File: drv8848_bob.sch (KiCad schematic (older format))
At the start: 1 part, among them J2 Conn_01x24

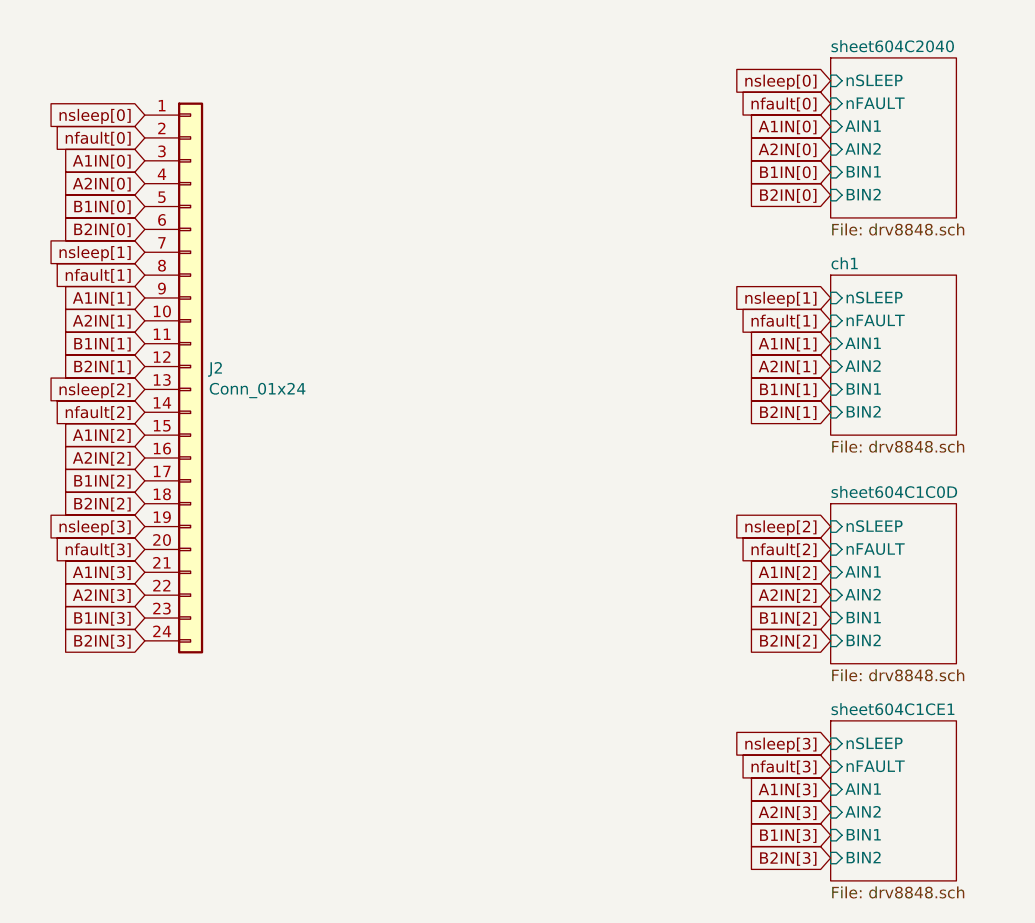
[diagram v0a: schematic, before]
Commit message: finalish
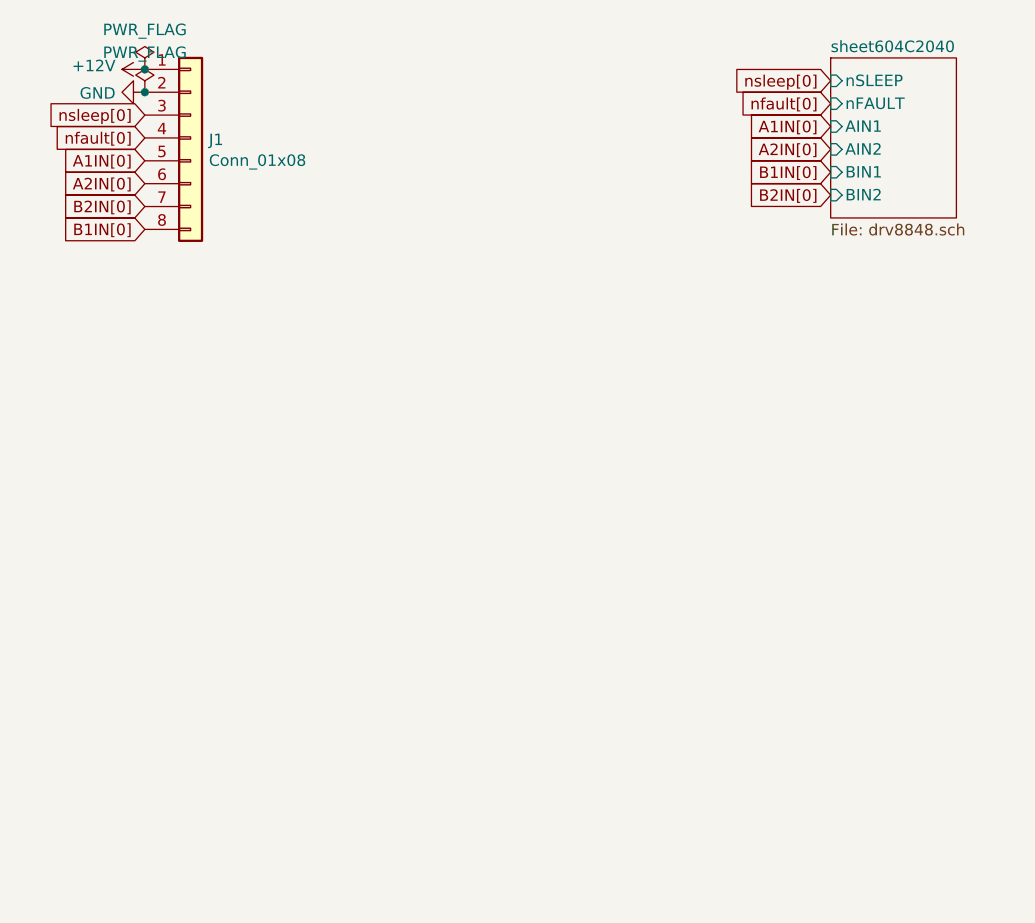
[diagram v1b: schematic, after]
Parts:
- removed J2: Conn_01x24, Connector_PinHeader_2.54mm:PinHeader_1x24_P2.54mm_Vertical, symbol Connector_Generic:Conn_01x24
- added J1: Conn_01x08, Connector_PinHeader_2.54mm:PinHeader_1x08_P2.54mm_Vertical, symbol Connector_Generic:Conn_01x08
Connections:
- net A1IN[0]: now also J1.5 (Pin_5)
- net A2IN[0]: now also J1.6 (Pin_6)
- net B1IN[0]: now also J1.8 (Pin_8)
- net B2IN[0]: now also J1.7 (Pin_7)
- net nfault[0]: now also J1.4 (Pin_4)
- net nsleep[0]: now also J1.3 (Pin_3)
- new net +12V: J1.1 (Pin_1)
- new net GND: J1.2 (Pin_2)
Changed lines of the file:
@@
 $Descr A4 11693 8268
 encoding utf-8
-Sheet 1 5
+Sheet 1 2
 Title ""
 Date ""
@@
 Comment4 ""
 $EndDescr
-$Sheet
-S 8900 2100 550  700
-U 604BEC61
-F0 "ch1" 50
-F1 "drv8848.sch" 50
-F2 "nSLEEP" I L 8900 2200 50
-F3 "nFAULT" I L 8900 2300 50
-F4 "AIN1" I L 8900 2400 50
-F5 "AIN2" I L 8900 2500 50
-F6 "BIN1" I L 8900 2600 50
-F7 "BIN2" I L 8900 2700 50
-$EndSheet
-$Sheet
-S 8900 3100 550  700
-U 604C1C15
-F0 "sheet604C1C0D" 50
-F1 "drv8848.sch" 50
-F2 "nSLEEP" I L 8900 3200 50
-F3 "nFAULT" I L 8900 3300 50
-F4 "AIN1" I L 8900 3400 50
-F5 "AIN2" I L 8900 3500 50
-F6 "BIN1" I L 8900 3600 50
-F7 "BIN2" I L 8900 3700 50
-$EndSheet
-$Sheet
-S 8900 4050 550  700
-U 604C1CE9
-F0 "sheet604C1CE1" 50
-F1 "drv8848.sch" 50
-F2 "nSLEEP" I L 8900 4150 50
-F3 "nFAULT" I L 8900 4250 50
-F4 "AIN1" I L 8900 4350 50
-F5 "AIN2" I L 8900 4450 50
-F6 "BIN1" I L 8900 4550 50
-F7 "BIN2" I L 8900 4650 50
-$EndSheet
 $Sheet
 S 8900 1150 550  700
@@
 Text GLabel 8900 1650 0    50   Input ~ 0
 B1IN[0]
-Text GLabel 8900 2200 0    50   Input ~ 0
-nsleep[1]
-Text GLabel 8900 2300 0    50   Input ~ 0
-nfault[1]
-Text GLabel 8900 2400 0    50   Input ~ 0
-A1IN[1]
-Text GLabel 8900 2500 0    50   Input ~ 0
-A2IN[1]
-Text GLabel 8900 2700 0    50   Input ~ 0
-B2IN[1]
-Text GLabel 8900 2600 0    50   Input ~ 0
-B1IN[1]
-Text GLabel 8900 3200 0    50   Input ~ 0
-nsleep[2]
-Text GLabel 8900 3300 0    50   Input ~ 0
-nfault[2]
-Text GLabel 8900 3400 0    50   Input ~ 0
-A1IN[2]
-Text GLabel 8900 3500 0    50   Input ~ 0
-A2IN[2]
-Text GLabel 8900 3700 0    50   Input ~ 0
-B2IN[2]
-Text GLabel 8900 3600 0    50   Input ~ 0
-B1IN[2]
-Text GLabel 8900 4150 0    50   Input ~ 0
-nsleep[3]
-Text GLabel 8900 4250 0    50   Input ~ 0
-nfault[3]
-Text GLabel 8900 4350 0    50   Input ~ 0
-A1IN[3]
-Text GLabel 8900 4450 0    50   Input ~ 0
-A2IN[3]
-Text GLabel 8900 4650 0    50   Input ~ 0
-B2IN[3]
-Text GLabel 8900 4550 0    50   Input ~ 0
-B1IN[3]
-$Comp
-L Connector_Generic:Conn_01x24 J2
-U 1 1 604C3E6E
-P 6100 2500
-F 0 "J2" H 6180 2492 50  0000 L CNN
-F 1 "Conn_01x24" H 6180 2401 50  0000 L CNN
-F 2 "Connector_PinHeader_2.54mm:PinHeader_1x24_P2.54mm_Vertical" H 6100 2500 50  0001 C CNN
-F 3 "~" H 6100 2500 50  0001 C CNN
-	1    6100 2500
-	1    0    0    -1
-$EndComp
 Text GLabel 5900 1400 0    50   Input ~ 0
 nsleep[0]
@@
 Text GLabel 5900 1700 0    50   Input ~ 0
 A2IN[0]
+Text GLabel 5900 1800 0    50   Input ~ 0
+B2IN[0]
 Text GLabel 5900 1900 0    50   Input ~ 0
-B2IN[0]
-Text GLabel 5900 1800 0    50   Input ~ 0
 B1IN[0]
-Text GLabel 5900 2000 0    50   Input ~ 0
-nsleep[1]
-Text GLabel 5900 2100 0    50   Input ~ 0
-nfault[1]
-Text GLabel 5900 2200 0    50   Input ~ 0
-A1IN[1]
-Text GLabel 5900 2300 0    50   Input ~ 0
-A2IN[1]
-Text GLabel 5900 2500 0    50   Input ~ 0
-B2IN[1]
-Text GLabel 5900 2400 0    50   Input ~ 0
-B1IN[1]
-Text GLabel 5900 2600 0    50   Input ~ 0
-nsleep[2]
-Text GLabel 5900 2700 0    50   Input ~ 0
-nfault[2]
-Text GLabel 5900 2800 0    50   Input ~ 0
-A1IN[2]
-Text GLabel 5900 2900 0    50   Input ~ 0
-A2IN[2]
-Text GLabel 5900 3100 0    50   Input ~ 0
-B2IN[2]
-Text GLabel 5900 3000 0    50   Input ~ 0
-B1IN[2]
-Text GLabel 5900 3200 0    50   Input ~ 0
-nsleep[3]
-Text GLabel 5900 3300 0    50   Input ~ 0
-nfault[3]
-Text GLabel 5900 3400 0    50   Input ~ 0
-A1IN[3]
-Text GLabel 5900 3500 0    50   Input ~ 0
-A2IN[3]
-Text GLabel 5900 3700 0    50   Input ~ 0
-B2IN[3]
-Text GLabel 5900 3600 0    50   Input ~ 0
-B1IN[3]
+$Comp
+L Connector_Generic:Conn_01x08 J1
+U 1 1 604D472A
+P 6100 1500
+F 0 "J1" H 6180 1492 50  0000 L CNN
+F 1 "Conn_01x08" H 6180 1401 50  0000 L CNN
+F 2 "Connector_PinHeader_2.54mm:PinHeader_1x08_P2.54mm_Vertical" H 6100 1500 50  0001 C CNN
+F 3 "~" H 6100 1500 50  0001 C CNN
+	1    6100 1500
+	1    0    0    -1
+$EndComp
+$Comp
+L power:GND #PWR02
+U 1 1 604D5DC7
+P 5900 1300
+F 0 "#PWR02" H 5900 1050 50  0001 C CNN
+F 1 "GND" V 5905 1172 50  0000 R CNN
+F 2 "" H 5900 1300 50  0001 C CNN
+F 3 "" H 5900 1300 50  0001 C CNN
+	1    5900 1300
+	0    1    1    0
+$EndComp
+$Comp
+L power:+12V #PWR01
+U 1 1 604D6180
+P 5900 1200
+F 0 "#PWR01" H 5900 1050 50  0001 C CNN
+F 1 "+12V" V 5915 1328 50  0000 L CNN
+F 2 "" H 5900 1200 50  0001 C CNN
+F 3 "" H 5900 1200 50  0001 C CNN
+	1    5900 1200
+	0    -1   -1   0
+$EndComp
+$Comp
+L power:PWR_FLAG #FLG0101
+U 1 1 604D6A4C
+P 5900 1200
+F 0 "#FLG0101" H 5900 1275 50  0001 C CNN
+F 1 "PWR_FLAG" H 5900 1373 50  0000 C CNN
+F 2 "" H 5900 1200 50  0001 C CNN
+F 3 "~" H 5900 1200 50  0001 C CNN
+	1    5900 1200
+	1    0    0    -1
+$EndComp
+Connection ~ 5900 1200
+$Comp
+L power:PWR_FLAG #FLG0102
+U 1 1 604D6A85
+P 5900 1300
+F 0 "#FLG0102" H 5900 1375 50  0001 C CNN
+F 1 "PWR_FLAG" H 5900 1473 50  0000 C CNN
+F 2 "" H 5900 1300 50  0001 C CNN
+F 3 "~" H 5900 1300 50  0001 C CNN
+	1    5900 1300
+	1    0    0    -1
+$EndComp
+Connection ~ 5900 1300
 $EndSCHEMATC
